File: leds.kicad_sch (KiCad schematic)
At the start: 20 parts

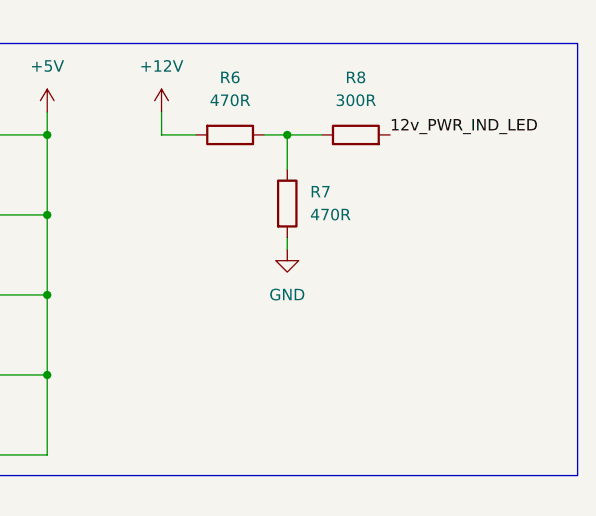
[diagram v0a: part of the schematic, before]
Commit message: Updated layout and schem
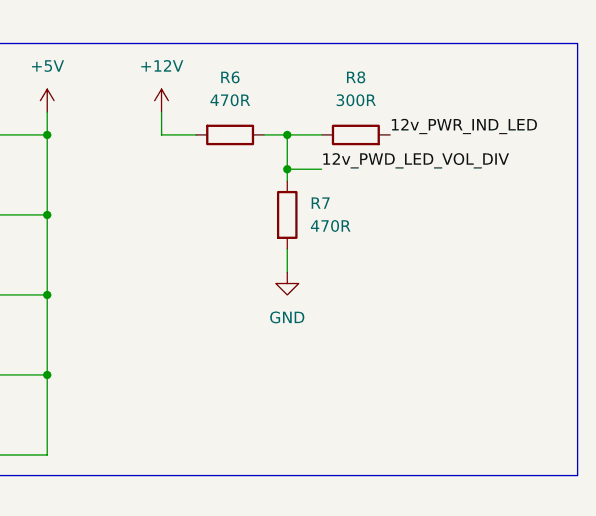
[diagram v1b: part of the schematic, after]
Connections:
- net 12v_PWD_LED_VOL_DIV: now reaches R6.1, R7.1, R8.1
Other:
- moved on the sheet: R7
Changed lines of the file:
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@@
+	)
+	(junction
+		(at 208.28 41.91)
+		(diameter 0)
+		(color 0 0 0 0)
 	)
 	(junction
@@
 	(wire
 		(pts
+			(xy 208.28 41.91) (xy 212.09 41.91)
+		)
+		(stroke
+			(width 0)
+			(type default)
+		)
+	)
+	(wire
+		(pts
 			(xy 173.99 38.1) (xy 181.61 38.1)
 		)
@@
 	(wire
 		(pts
-			(xy 208.28 41.91) (xy 208.28 38.1)
+			(xy 208.28 43.18) (xy 208.28 41.91)
 		)
 		(stroke
@@
 	(wire
 		(pts
-			(xy 208.28 49.53) (xy 208.28 50.8)
+			(xy 208.28 50.8) (xy 208.28 53.34)
 		)
 		(stroke
@@
 		(pts
 			(xy 129.54 35.56) (xy 129.54 46.99)
+		)
+		(stroke
+			(width 0)
+			(type default)
+		)
+	)
+	(wire
+		(pts
+			(xy 208.28 38.1) (xy 208.28 41.91)
 		)
 		(stroke
@@
 	(label "PUMP_PWM_IND_LED_5v"
 		(at 52.07 66.04 0)
+		(fields_autoplaced yes)
+		(effects
+			(font
+				(size 1.27 1.27)
+			)
+			(justify left bottom)
+		)
+	)
+	(label "12v_PWD_LED_VOL_DIV"
+		(at 212.09 41.91 0)
 		(fields_autoplaced yes)
 		(effects
@@
 	(symbol
 		(lib_id "Device:R")
-		(at 208.28 45.72 0)
+		(at 208.28 46.99 0)
 		(unit 1)
 		(exclude_from_sim no)
@@
 		(fields_autoplaced yes)
 		(property "Reference" "R7"
-			(at 210.82 44.4499 0)
+			(at 210.82 45.7199 0)
 			(effects
 				(font
@@
 		)
 		(property "Value" "470R"
-			(at 210.82 46.9899 0)
+			(at 210.82 48.2599 0)
 			(effects
 				(font
@@
 		)
 		(property "Footprint" "Resistor_SMD:R_0805_2012Metric"
-			(at 206.502 45.72 90)
+			(at 206.502 46.99 90)
 			(effects
 				(font
@@
 		)
 		(property "Datasheet" "~"
-			(at 208.28 45.72 0)
+			(at 208.28 46.99 0)
 			(effects
 				(font
@@
 		)
 		(property "Description" "Resistor"
-			(at 208.28 45.72 0)
+			(at 208.28 46.99 0)
 			(effects
 				(font
@@
 	(symbol
 		(lib_id "power:GND")
-		(at 208.28 50.8 0)
+		(at 208.28 53.34 0)
 		(unit 1)
 		(exclude_from_sim no)
@@
 		(fields_autoplaced yes)
 		(property "Reference" "#PWR049"
-			(at 208.28 57.15 0)
+			(at 208.28 59.69 0)
 			(effects
 				(font
@@
 		)
 		(property "Value" "GND"
-			(at 208.28 55.88 0)
+			(at 208.28 58.42 0)
 			(effects
 				(font
@@
 		)
 		(property "Footprint" ""
-			(at 208.28 50.8 0)
+			(at 208.28 53.34 0)
 			(effects
 				(font
@@
 		)
 		(property "Datasheet" ""
-			(at 208.28 50.8 0)
+			(at 208.28 53.34 0)
 			(effects
 				(font
@@
 		)
 		(property "Description" "Power symbol creates a global label with name \"GND\" , ground"
-			(at 208.28 50.8 0)
-			(effects
-				(font
+			(at 208.28 53.34 0)
+			(effects
+				(font
